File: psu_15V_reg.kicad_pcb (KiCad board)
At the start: 2 copper layers, 18 parts, among them J1 IN, J2 OUT, U1 LM317_TO-252, U2 LM337_TO252

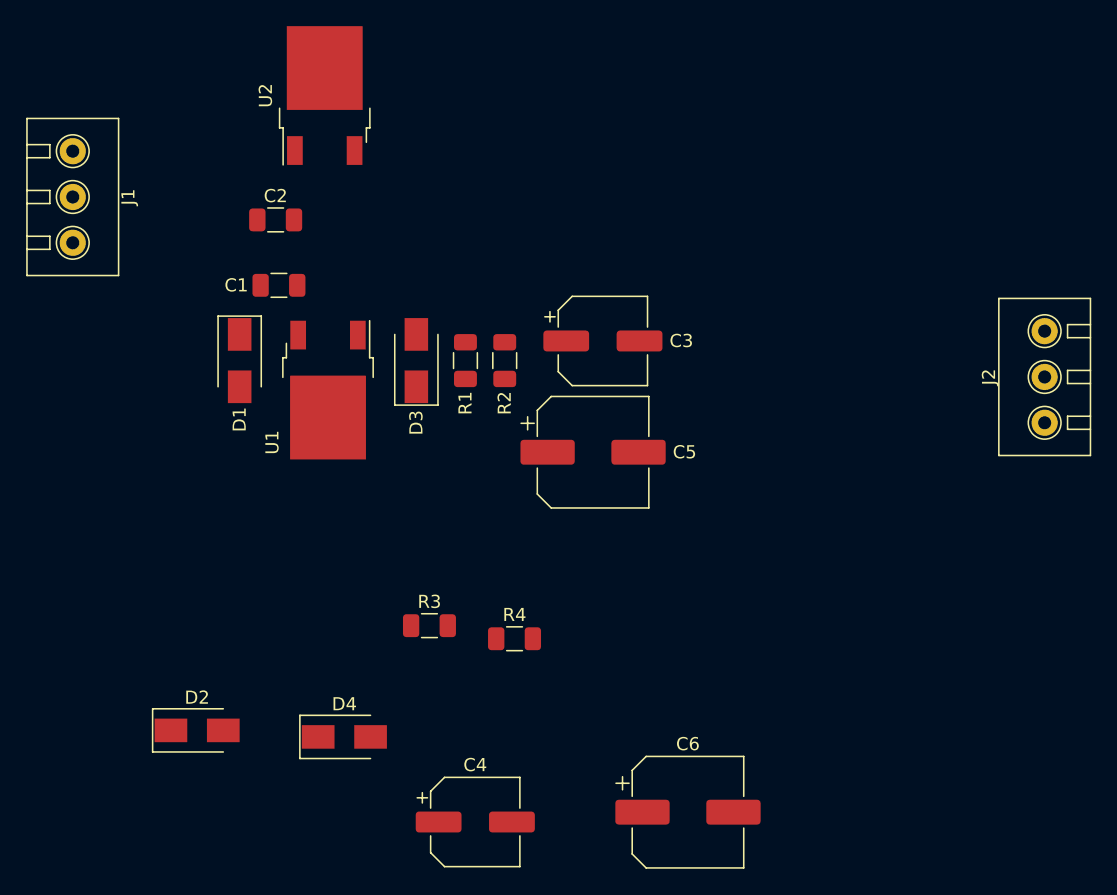
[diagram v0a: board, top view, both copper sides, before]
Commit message: progressing
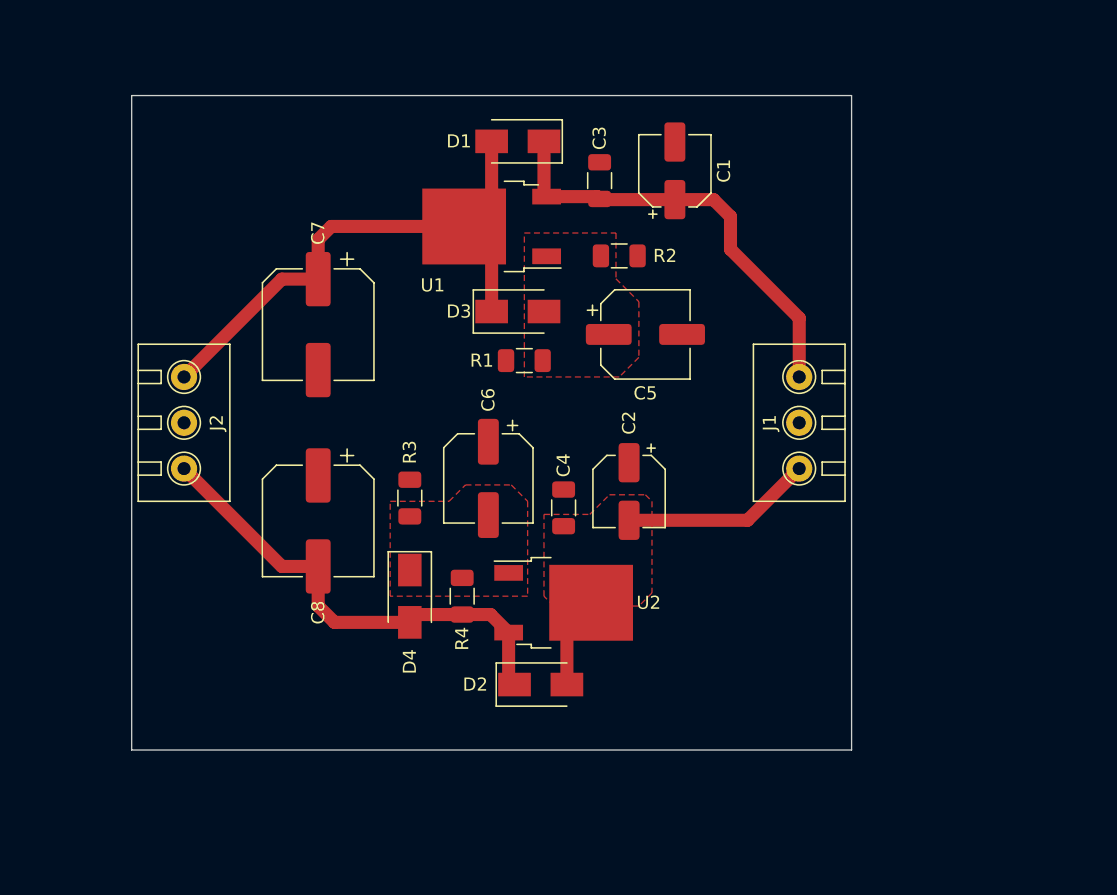
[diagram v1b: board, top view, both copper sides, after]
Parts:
- added C1: 10uF, Capacitor_SMD:CP_Elec_5x5.3, F.Cu at (146.5, 83.2)
- added C2: 10uF, Capacitor_SMD:CP_Elec_5x5.3, F.Cu at (143.0, 107.8)
- moved J2 65.8 mm to (109.0, 102.5), turned to 270 degrees
- moved J1 58.1 mm to (156.0, 102.5), turned to 90 degrees
- moved U2 42.8 mm to (138.0, 116.2), turned to 0 degrees
- moved C8 36.0 mm to (119.2, 110.0), turned to 270 degrees
- moved C4 31.1 mm to (138.0, 109.0), turned to 270 degrees
- moved D1 27.1 mm to (134.5, 81.0), turned to 180 degrees
- moved D2 26.5 mm to (136.2, 122.5)
- moved C6 26.3 mm to (132.2, 106.8), turned to 270 degrees
- moved C3 25.8 mm to (140.8, 84.0), turned to 90 degrees
- moved C7 23.2 mm to (119.2, 95.0), turned to 270 degrees
- moved U1 17.7 mm to (132.5, 87.5), turned to 180 degrees
- moved D4 11.9 mm to (126.2, 115.8), turned to 270 degrees
- moved R2 11.9 mm to (142.2, 89.8), turned to 0 degrees
- moved R3 9.86 mm to (126.2, 108.2), turned to 270 degrees
- moved D3 8.61 mm to (134.5, 94.0), turned to 0 degrees
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- renumbered C1 to C3, C2 to C4, C3 to C5, C4 to C6, C5 to C7, C6 to C8
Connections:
- J2 pad 1: /VO- -> /VO+
- J2 pad 3: /VO+ -> /VO-
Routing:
- net /VO+: track 0.00 -> 42.7 mm
- net /VO-: track 0.00 -> 36.4 mm
- net /VI+: track 0.00 -> 33.4 mm
- net /VI-: track 0.00 -> 21.7 mm
- added copper zone on F.Cu, net /ADJ+
- added copper zone on F.Cu, net /ADJ-
- added copper zone on F.Cu, net /VI-
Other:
- board outline added: 55 x 50 mm
